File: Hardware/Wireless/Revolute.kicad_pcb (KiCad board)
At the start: 4 copper layers, 19.8 x 20 mm, 57 parts, among them U1 BQ27441-G1, U2 nrf52833_qfn40, U3 AS5600, U4 AP2112K-3.3, U5 BQ24075RGT, U6 Button, X1 32.768 kHz, X2 32MHZ

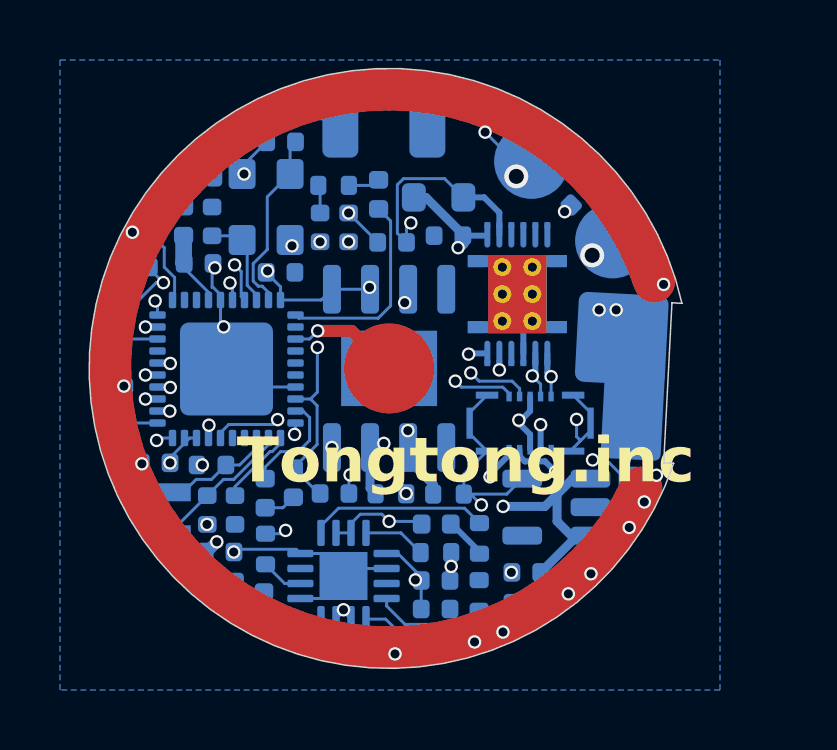
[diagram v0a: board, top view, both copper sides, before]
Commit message: updated gerbers
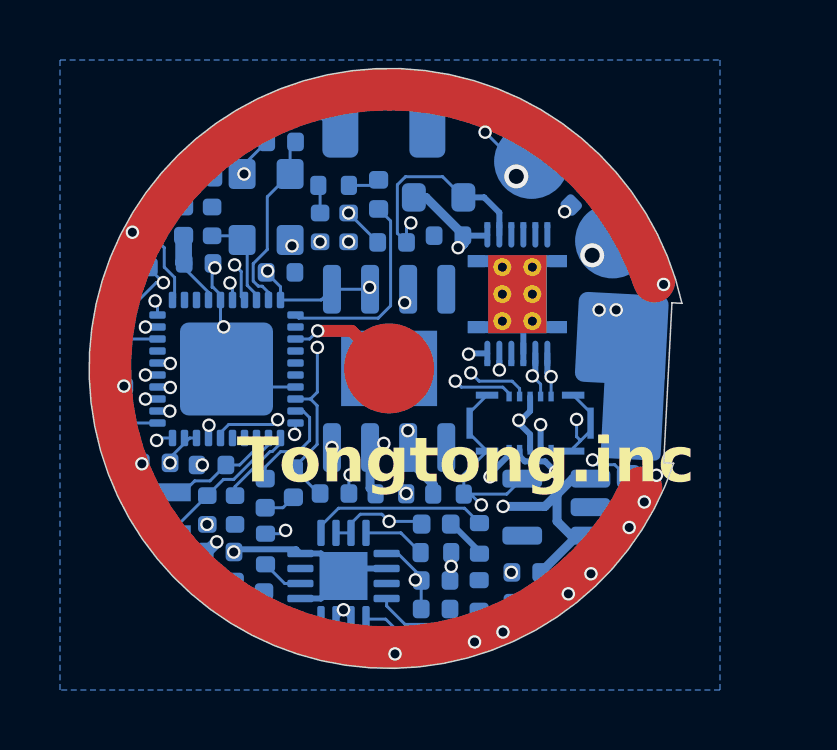
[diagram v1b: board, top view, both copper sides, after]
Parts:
- moved ? 0.08 mm to (179.0, 98.6)
